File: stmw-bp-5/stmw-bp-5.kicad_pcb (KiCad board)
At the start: 2 copper layers, 100 x 86 mm, 11 parts, among them J1 Conn_02x25_Odd_Even, J2 Conn_02x25_Odd_Even, U1 X1611WVS-98-9TV01, U2 X1611WVS-98-9TV01, U3 X1611WVS-98-9TV01, U4 X1611WVS-98-9TV01, U5 X1611WVS-98-9TV01

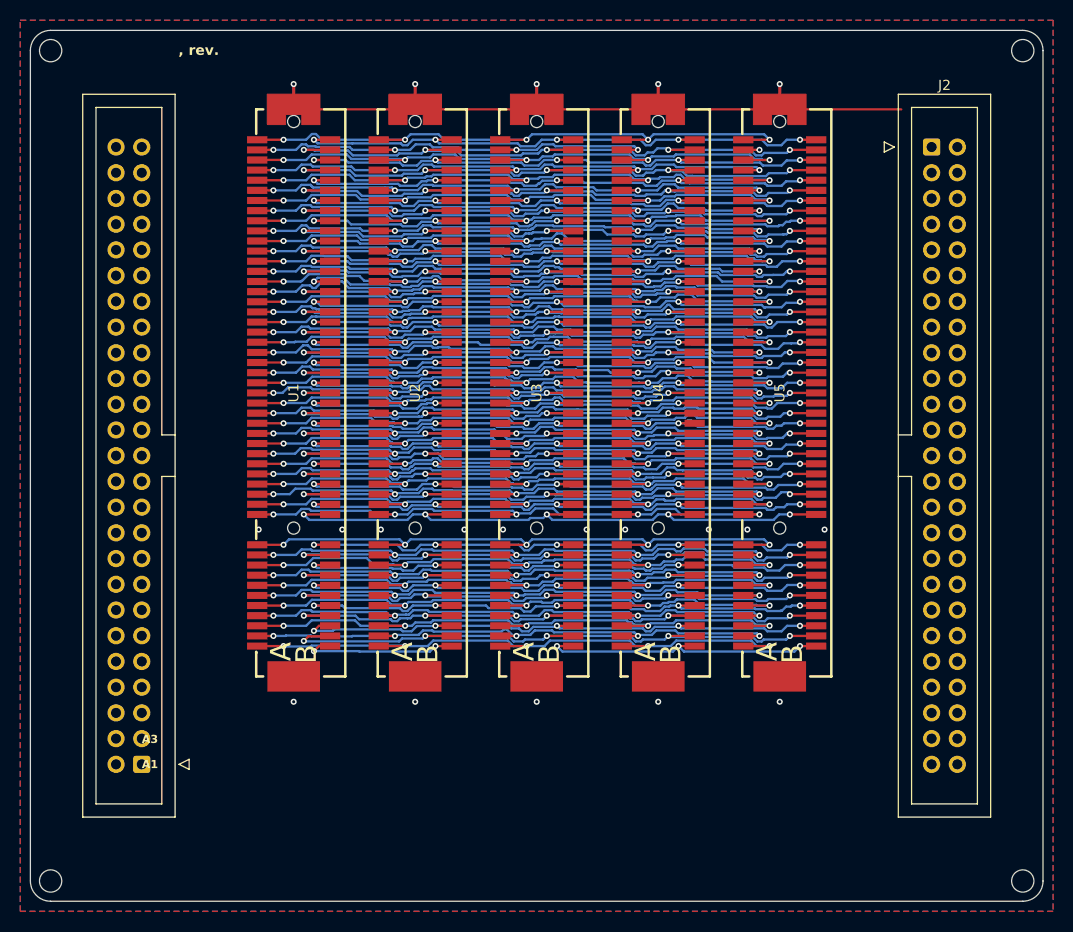
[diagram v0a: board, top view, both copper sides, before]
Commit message: Hmmmm
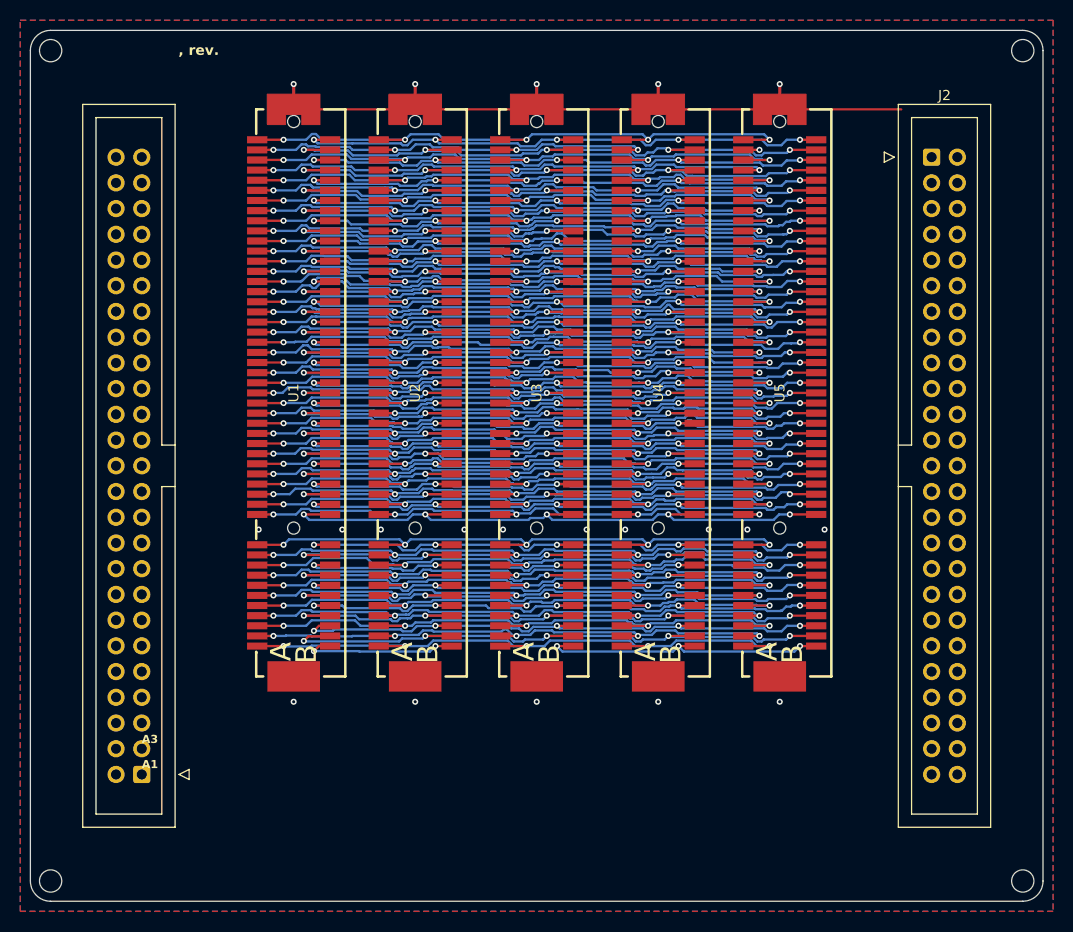
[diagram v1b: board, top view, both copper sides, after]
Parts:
- moved J1 1.00 mm to (101.0, 113.5)
- moved J2 1.00 mm to (179.0, 52.5)
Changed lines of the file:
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@@
 	(property "COMPANY" "STM32World")
 	(property "REVISION" "a")
-	(property "TITLE" "STMW-BP-6")
+	(property "TITLE" "STMW-BP-5")
 	(net 0 "")
 	(net 1 "B1")
@@
 		)
 		(sheetname "/")
-		(sheetfile "bp.kicad_sch")
+		(sheetfile "stmw-bp-5.kicad_sch")
 		(attr smd)
 		(fp_line
@@
 		)
 		(sheetname "/")
-		(sheetfile "bp.kicad_sch")
+		(sheetfile "stmw-bp-5.kicad_sch")
 		(attr smd)
 		(fp_line
@@
 		(property ki_fp_filters "MountingHole*")
 		(sheetname "/")
-		(sheetfile "bp.kicad_sch")
+		(sheetfile "stmw-bp-5.kicad_sch")
 		(attr exclude_from_pos_files exclude_from_bom)
 		(fp_circle
@@
 		)
 		(sheetname "/")
-		(sheetfile "bp.kicad_sch")
+		(sheetfile "stmw-bp-5.kicad_sch")
 		(attr smd)
 		(fp_line
@@
 	(footprint "Connector_IDC:IDC-Header_2x25_P2.54mm_Vertical"
 		(layer "F.Cu")
-		(at 179 51.52)
+		(at 179 52.52)
 		(descr "Through hole IDC box header, 2x25, 2.54mm pitch, DIN 41651 / IEC 60603-13, double rows, https://docs.google.com/spreadsheets/d/16SsEcesNF15N3Lb4niX7dcUr-NY5_MFPQhobNuNppn4/edit#gid=0")
 		(tags "Through hole vertical IDC box header THT 2x25 2.54mm double row")
@@
 		(property ki_fp_filters "Connector*:*_2x??_*")
 		(sheetname "/")
-		(sheetfile "bp.kicad_sch")
+		(sheetfile "stmw-bp-5.kicad_sch")
 		(attr through_hole)
 		(fp_line
@@
 		)
 		(sheetname "/")
-		(sheetfile "bp.kicad_sch")
+		(sheetfile "stmw-bp-5.kicad_sch")
 		(attr smd)
 		(fp_line
@@
 		(property ki_fp_filters "MountingHole*")
 		(sheetname "/")
-		(sheetfile "bp.kicad_sch")
+		(sheetfile "stmw-bp-5.kicad_sch")
 		(attr exclude_from_pos_files exclude_from_bom)
 		(fp_circle
@@
 		(property ki_fp_filters "MountingHole*")
 		(sheetname "/")
-		(sheetfile "bp.kicad_sch")
+		(sheetfile "stmw-bp-5.kicad_sch")
 		(attr exclude_from_pos_files exclude_from_bom)
 		(fp_circle
@@
 		)
 		(sheetname "/")
-		(sheetfile "bp.kicad_sch")
+		(sheetfile "stmw-bp-5.kicad_sch")
 		(attr smd)
 		(fp_line
@@
 	(footprint "Connector_IDC:IDC-Header_2x25_P2.54mm_Vertical"
 		(layer "F.Cu")
-		(at 101 112.48 180)
+		(at 101 113.48 180)
 		(descr "Through hole IDC box header, 2x25, 2.54mm pitch, DIN 41651 / IEC 60603-13, double rows, https://docs.google.com/spreadsheets/d/16SsEcesNF15N3Lb4niX7dcUr-NY5_MFPQhobNuNppn4/edit#gid=0")
 		(tags "Through hole vertical IDC box header THT 2x25 2.54mm double row")
@@
 		(property ki_fp_filters "Connector*:*_2x??_*")
 		(sheetname "/")
-		(sheetfile "bp.kicad_sch")
+		(sheetfile "stmw-bp-5.kicad_sch")
 		(attr through_hole)
 		(fp_line
@@
 		(property ki_fp_filters "MountingHole*")
 		(sheetname "/")
-		(sheetfile "bp.kicad_sch")
+		(sheetfile "stmw-bp-5.kicad_sch")
 		(attr exclude_from_pos_files exclude_from_bom)
 		(fp_circle
@@
 	)
 	(gr_line
-		(start 83 82)
-		(end 203 82)
+		(start 83 83)
+		(end 203 83)
 		(stroke
 			(width 0.1)
@@
 		(layer "Dwgs.User")
 		(pts
+			(xy 90 126) (xy 90 83)
+		)
+		(height -4)
+		(orientation 1)
+		(format
+			(prefix "")
+			(suffix "")
+			(units 3)
+			(units_format 1)
+			(precision 4)
+		)
+		(style
+			(thickness 0.1)
+			(arrow_length 1.27)
+			(text_position_mode 0)
+			(arrow_direction outward)
+			(extension_height 0.58642)
+			(extension_offset 0.5)
+			(keep_text_aligned yes)
+		)
+		(gr_text "43.0000 mm"
+			(at 84.85 104.5 90)
+			(layer "Dwgs.User")
+			(effects
+				(font
+					(size 1 1)
+					(thickness 0.15)
+				)
+			)
+		)
+	)
+	(dimension
+		(type orthogonal)
+		(layer "Dwgs.User")
+		(pts
 			(xy 190 40) (xy 90 40)
 		)
-		(height -3)
+		(height -10)
 		(orientation 0)
 		(format
@@
 		)
 		(gr_text "100.0000 mm"
-			(at 140 35.85 0)
+			(at 140 28.85 0)
 			(layer "Dwgs.User")
 			(effects
@@
 			(xy 90 126) (xy 90 40)
 		)
-		(height -5)
+		(height -6)
 		(orientation 1)
 		(format
@@
 		)
 		(gr_text "86.0000 mm"
-			(at 83.85 83 90)
+			(at 82.85 83 90)
 			(layer "Dwgs.User")
 			(effects
@@
 		(min_thickness 0.127)
 		(filled_areas_thickness no)
-		(fill
+		(fill yes
 			(thermal_gap 0.127)
 			(thermal_bridge_width 0.254)
